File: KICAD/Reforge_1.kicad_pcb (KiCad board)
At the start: 2 copper layers, 66.5 x 80.4 mm, 87 parts, among them J1 USB_C_Receptacle_USB2.0_16P, J10 Conn_01x14_Pin, J11 Conn_01x12_Pin, J12 Conn_01x12_Pin, J14 Conn_01x12_Pin, J15 Conn_01x12_Pin, J3 Conn_01x02, J8 Conn_01x12_Pin, J9 Conn_01x14_Pin, Q1 SS8050, Q2 SS8050, SW1 SW_Push, SW2 SW_Push, U11 SN74LVC2G125DCUR, U2 CP2102N-Axx-xQFN28, U3 ICE40UP5K-SG48ITR, U4 AP2112K-1.2, U5 ESP32-WROOM-32D, U6 AMS1117-3.3, U8 W25Q32JVSS, Y1 SG-210STF

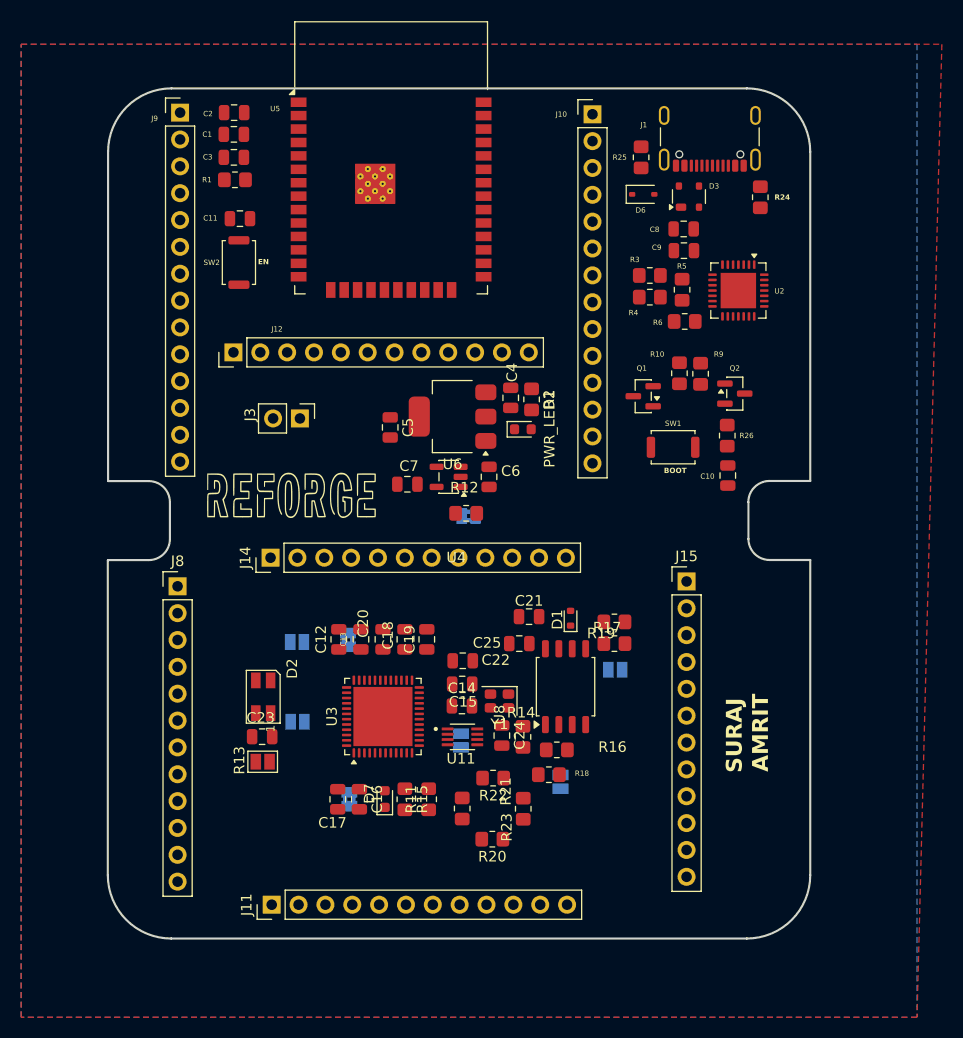
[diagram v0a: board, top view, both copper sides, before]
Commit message: UPDATED PCB
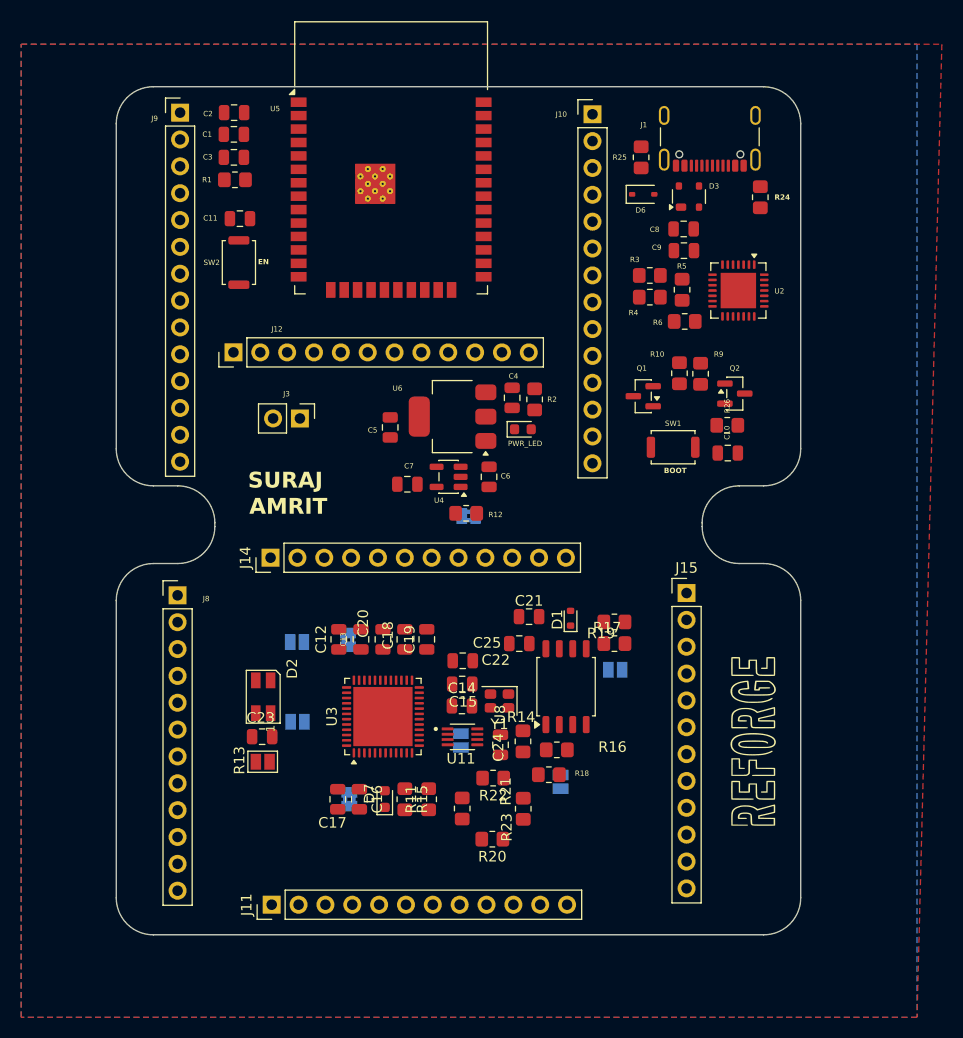
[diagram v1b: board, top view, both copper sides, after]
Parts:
- moved G*** 50.0 mm to (167.7, 108.7), turned to 90 degrees
- moved C10 2.12 mm to (163.6, 81.6), turned to 0 degrees
- moved J15 1.09 mm to (159.7, 94.9)
- moved R26 0.97 mm to (163.5, 79.0), turned to 0 degrees
- moved C24 0.88 mm to (142.1, 109.2)
- moved J8 0.85 mm to (111.5, 95.1)
- moved R14 0.43 mm to (144.2, 108.9)
- moved R2 0.29 mm to (145.3, 76.5)
- moved C4 0.14 mm to (143.2, 76.4)
- moved U8 0.05 mm to (148.3, 103.7)
- renumbered PWR_LED1 to PWR_LED
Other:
- board size 66.5 x 80.4 mm -> 64.8 x 80.2 mm
